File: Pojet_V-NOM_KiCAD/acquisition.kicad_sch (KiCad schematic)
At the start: 7 parts, among them J3 Conn_01x08, J4 Conn_01x03, J5 Conn_01x03, U2 ADXL343

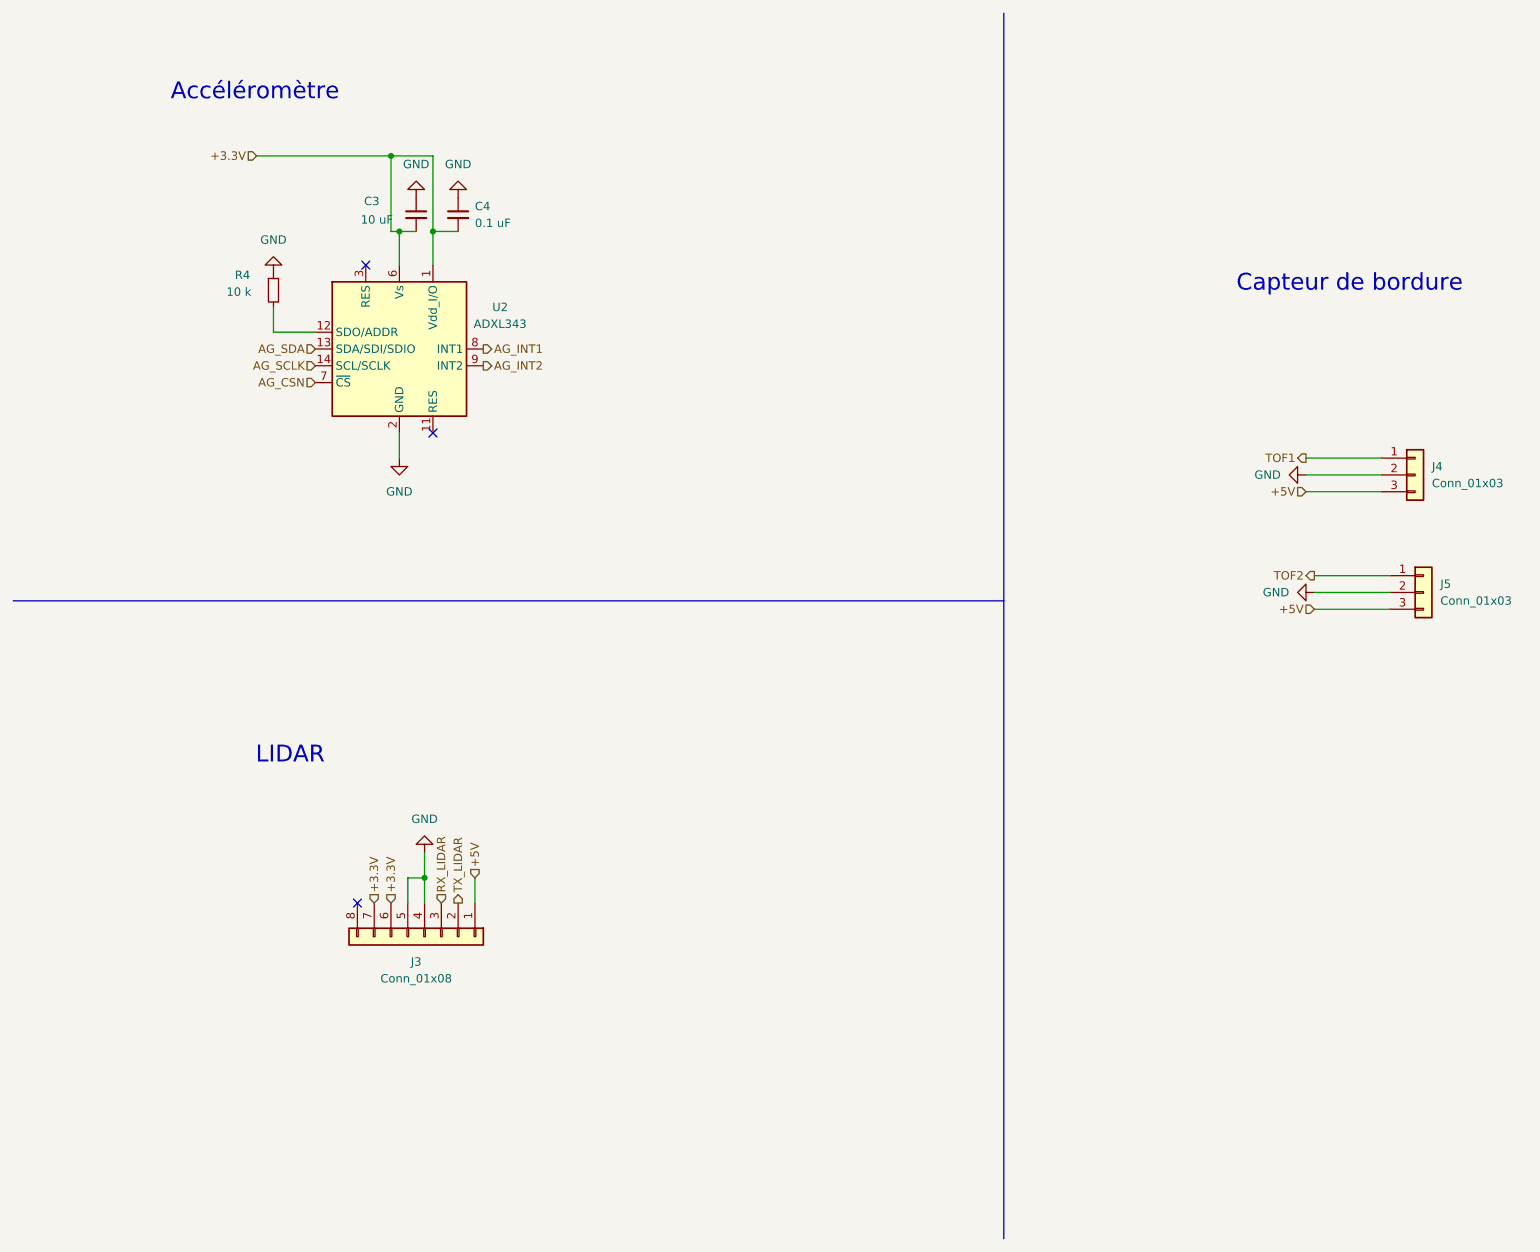
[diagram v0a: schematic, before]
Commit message: Retouches lisibilité Alim / capteurs
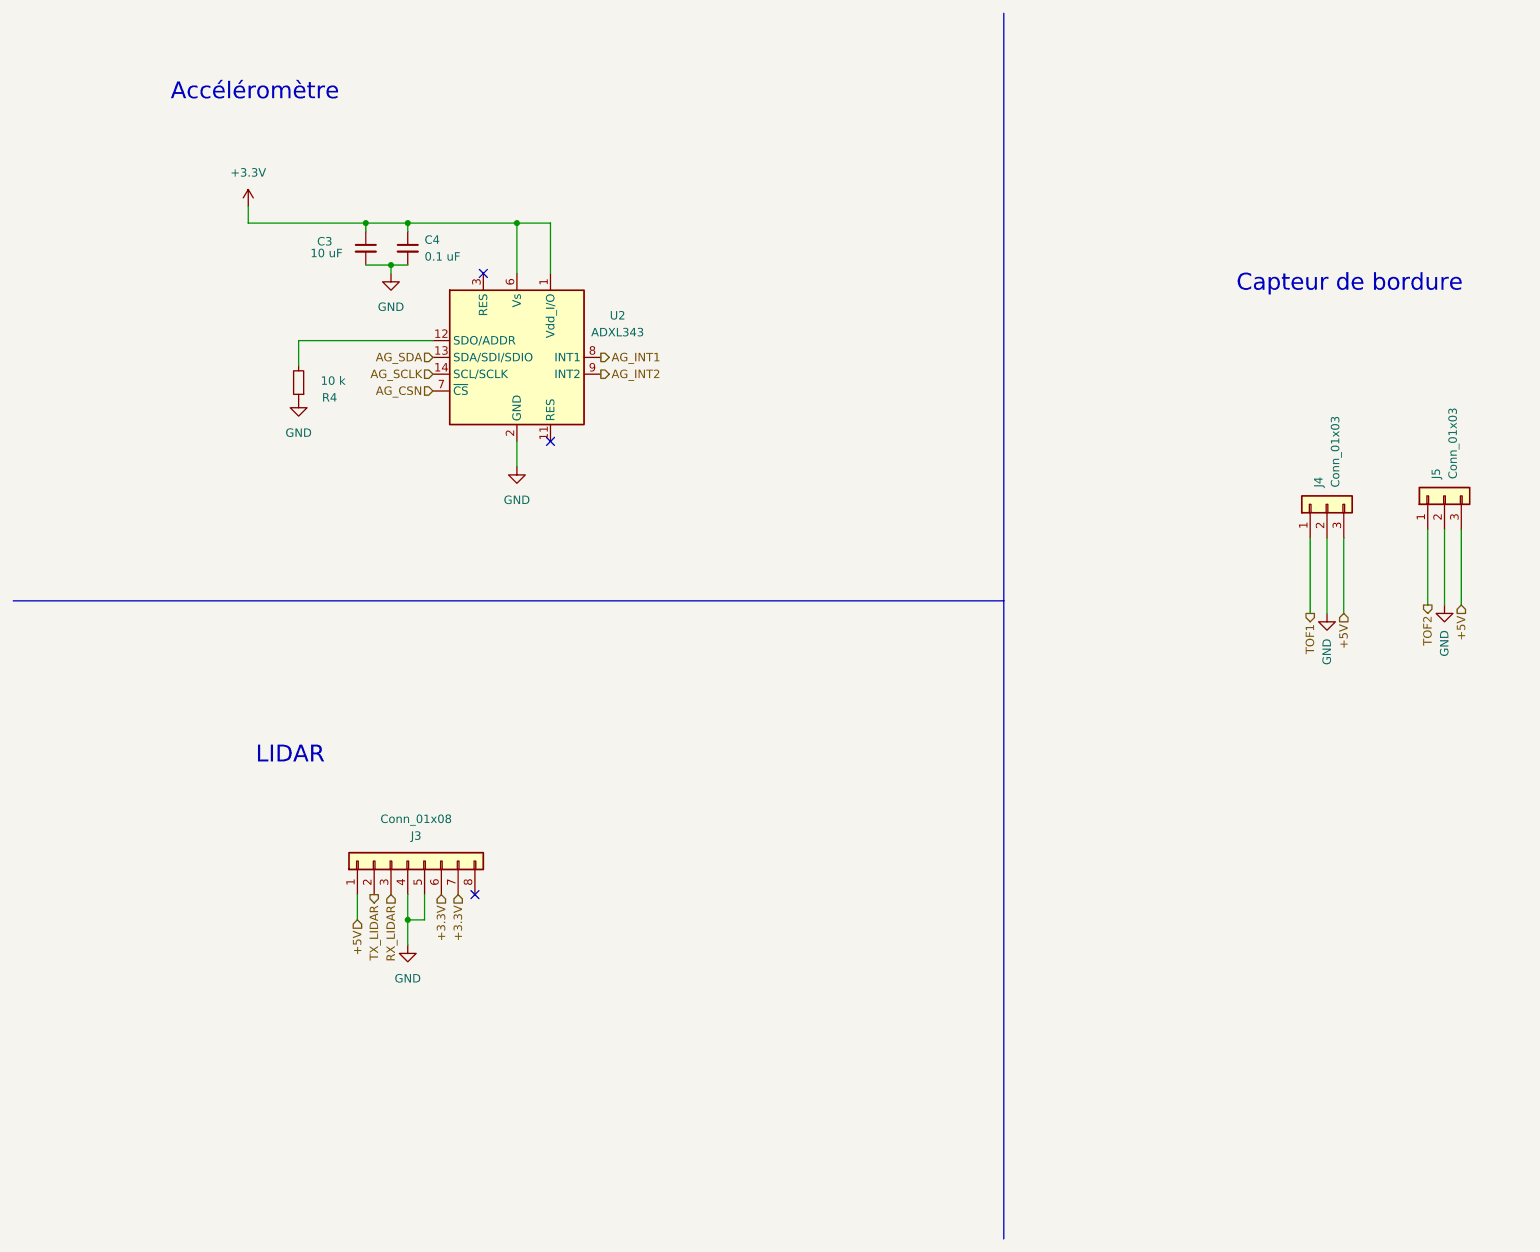
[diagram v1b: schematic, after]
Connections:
- net +3.3V: now also C3.1, C4.1; no longer C3.2, C4.2
- net GND: now also C3.2, C4.2; no longer C3.1, C4.1
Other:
- moved on the sheet: C3, C4, J3, J4, J5, R4, U2
